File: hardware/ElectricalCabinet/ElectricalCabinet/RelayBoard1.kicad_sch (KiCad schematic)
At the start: 0 parts

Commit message: Cabinet Schematics Update
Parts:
- added C1: 0.1uF, Capacitor_SMD:C_0805_2012Metric, symbol Device:C
- added D1, D2, D3, D4, D5, D6, D7, D8: LED, LED_SMD:LED_0805_2012Metric, symbol Device:LED
- added J1: Screw_Terminal_01x09, TerminalBlock:TerminalBlock_MaiXu_MX126-5.0-09P_1x09_P5.00mm, symbol Connector:Screw_Terminal_01x09
- added J2: Screw_Terminal_01x06, TerminalBlock:TerminalBlock_MaiXu_MX126-5.0-06P_1x06_P5.00mm, symbol Connector:Screw_Terminal_01x06
- added K1, K2, K3, K4, K5, K6, K7, K8: G3MB-202P DC5, TrafficLightLibrary:G3MB_202P_DC5, symbol TrafficLightLibrary:G3MB-202P_DC5
- added R1, R2, R3, R4, R5, R6, R7, R8: 1kΩ, Resistor_SMD:R_0805_2012Metric, symbol Device:R
- added U2: TPIC6B595N, TrafficLightLibrary:TPIC6B595N, symbol TrafficLightLibrary:TPIC6B595N
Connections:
- new net: C1.1, J2.2 (Pin_2), U2.10 (GND), U2.11 (GND), U2.19 (GND), U2.9 (~{G})
- new net: J2.4 (Pin_4), U2.12 (RCK)
- new net: J2.3 (Pin_3), U2.13 (SRCK)
- new net: K5.4, R5.2, U2.14 (DRAIN4)
- new net: K6.4, R6.2, U2.15 (DRAIN5)
- new net: K7.4, R7.2, U2.16 (DRAIN6)
- new net: K8.4, R8.2, U2.17 (DRAIN7)
- new net: J2.1 (Pin_1), U2.18 (SEROUT)
- new net: C1.2, J2.6 (Pin_6), U2.2 (VCC), U2.8 (~{SRCLR})
- new net: K1.4, R1.2, U2.4 (DRAIN0)
- new net: K2.4, R2.2, U2.5 (DRAIN1)
- new net: K3.4, R3.2, U2.6 (DRAIN2)
- new net: K4.4, R4.2, U2.7 (DRAIN3)
- new net: J1.5 (Pin_5), K5.2
- new net: D1.2 (A), D2.2 (A), D3.2 (A), D4.2 (A), D5.2 (A), D6.2 (A), D7.2 (A), D8.2 (A), K1.3, K2.3, K3.3, K4.3, K5.3, K6.3, K7.3, K8.3
- new net: J1.7 (Pin_7), K7.2
- new net: J1.4 (Pin_4), K4.2
- new net: D7.1 (K), R7.1
- new net: D8.1 (K), R8.1
- new net: D6.1 (K), R6.1
- new net: J1.3 (Pin_3), K3.2
- new net: D5.1 (K), R5.1
- new net: D3.1 (K), R3.1
- new net: D4.1 (K), R4.1
- new net: D1.1 (K), R1.1
- new net: J1.1 (Pin_1), K1.2
- new net: J1.2 (Pin_2), K2.2
- new net: J1.6 (Pin_6), K6.2
- new net: J1.8 (Pin_8), K8.2
- new net: D2.1 (K), R2.1
- new net 110vAC Hawt: J1.9 (Pin_9), K1.1, K2.1, K3.1, K4.1, K5.1, K6.1, K7.1, K8.1
- new net SERIN: J2.5 (Pin_5), U2.3 (SERIN)
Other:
- note added: "110vAC Hawt"

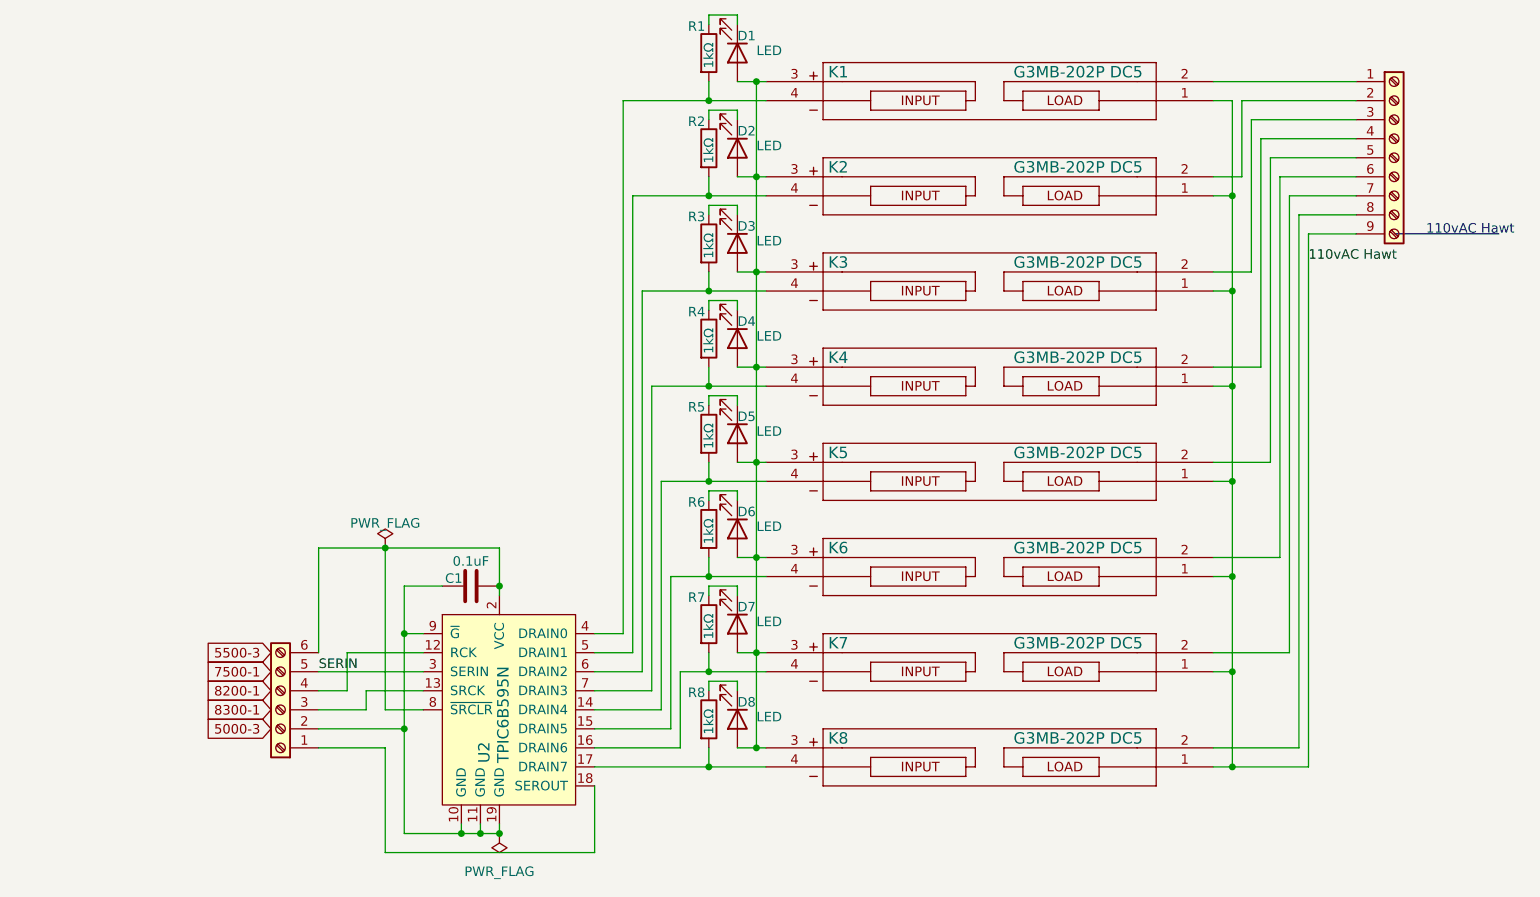
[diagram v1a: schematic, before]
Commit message: More updates
Added drawing sheets, wire label scheme, signal list, and traffic light label image to docs folder
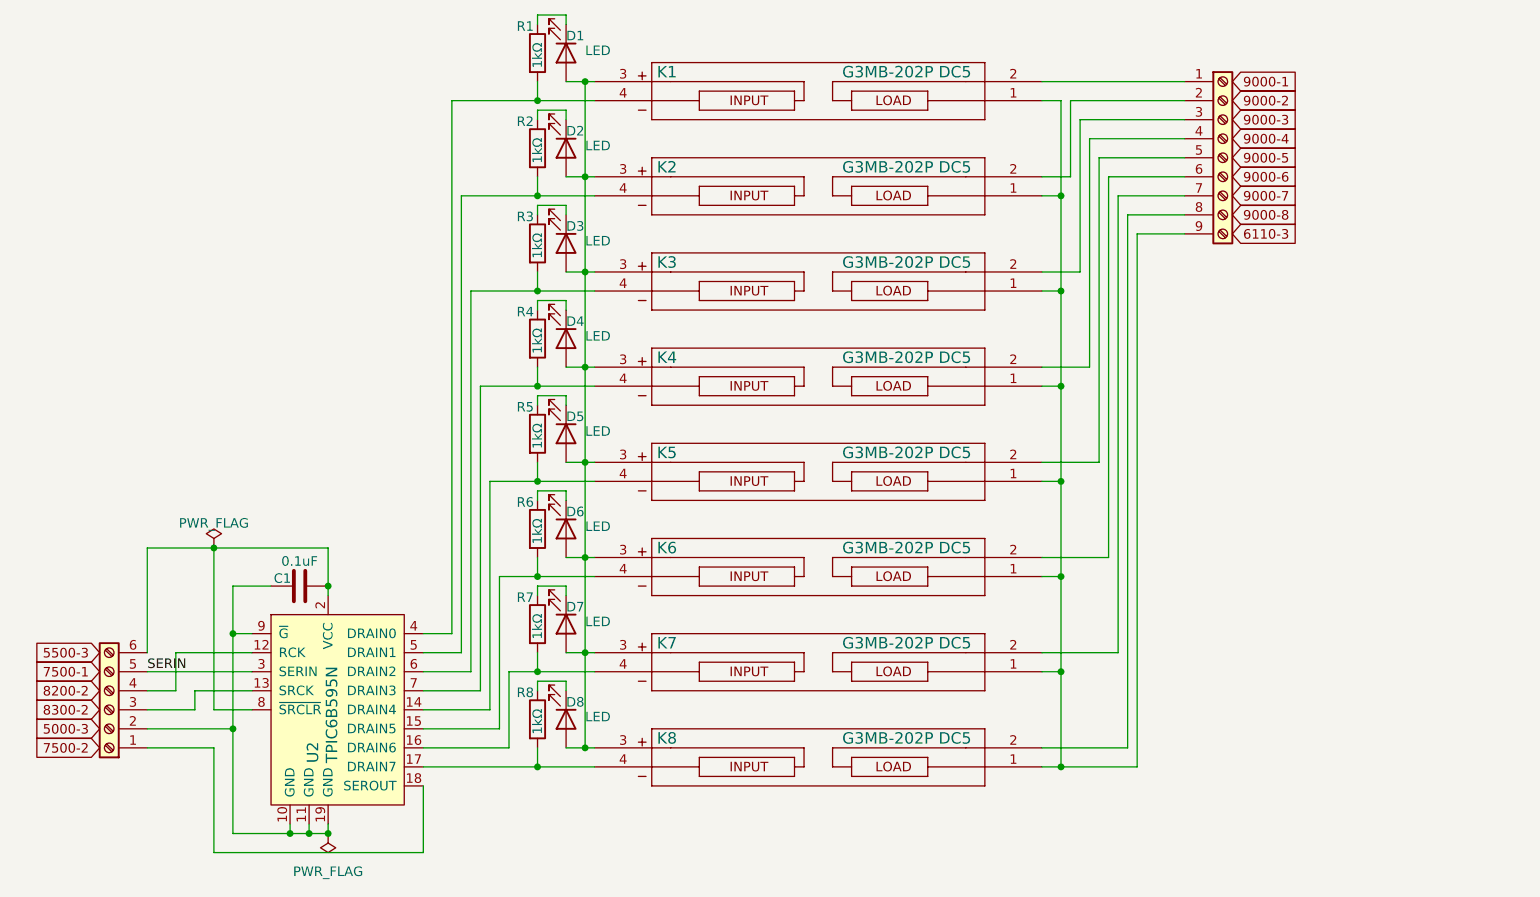
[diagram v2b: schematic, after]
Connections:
- net 110vAC Hawt: no longer names the net of J1.9 (Pin_9), K1.1, K2.1, K3.1, K4.1, K5.1, K6.1, K7.1, K8.1
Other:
- note removed: "110vAC Hawt"
- moved on the sheet: C1, D1, D2, D3, D4, D5, D6, D7, D8, K1, K2, K3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
